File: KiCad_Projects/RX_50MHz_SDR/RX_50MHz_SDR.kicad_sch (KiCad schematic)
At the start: 0 parts

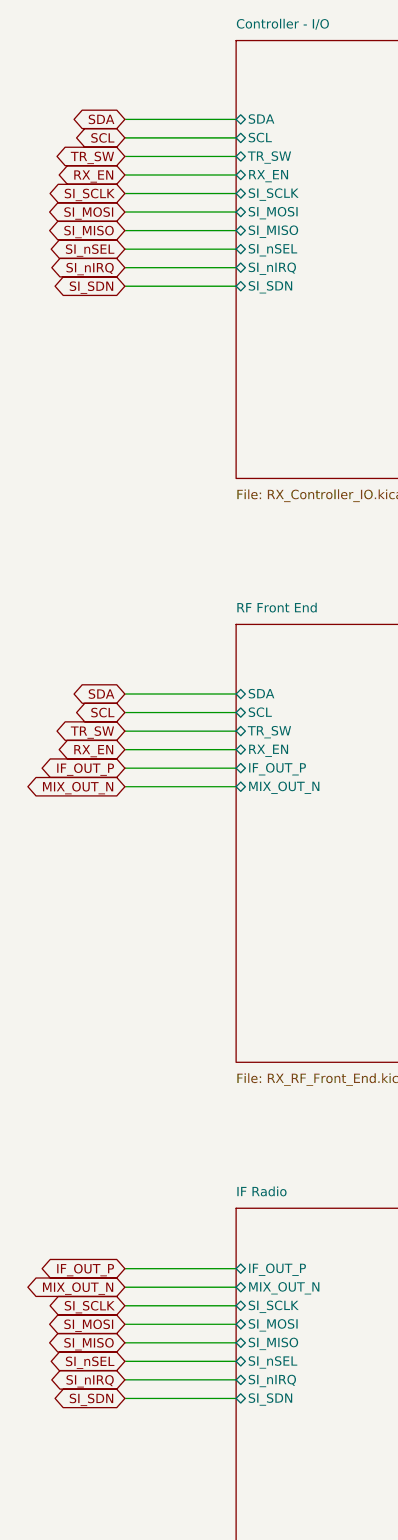
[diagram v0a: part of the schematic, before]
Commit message: lable correctly, local nets connected
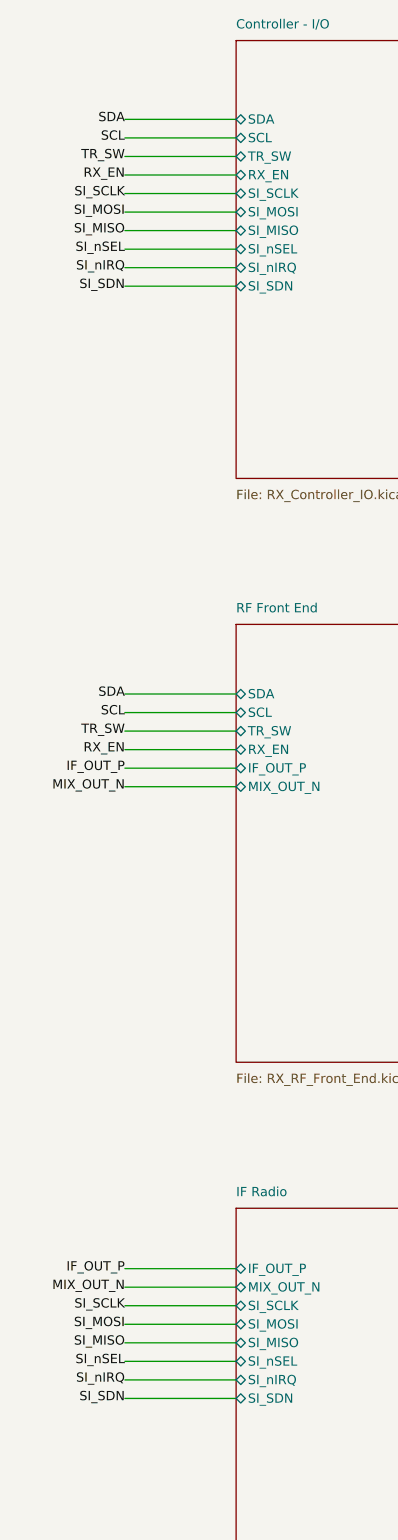
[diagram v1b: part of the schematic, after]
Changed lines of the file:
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@@
 	)
 	(wire (pts (xy 459.74 50.80) (xy 444.5 50.80)) (stroke (width 0) (type default)))
-	(global_label "SDA" (shape bidirectional) (at 444.5 50.80 180) (fields_autoplaced yes) (effects (font (size 1.27 1.27)) (justify right)))
+	(label "SDA"
+		(at 444.5 50.80 180)
+		(effects (font (size 1.27 1.27)) (justify right))
+	)
 	(wire (pts (xy 459.74 53.34) (xy 444.5 53.34)) (stroke (width 0) (type default)))
-	(global_label "SCL" (shape bidirectional) (at 444.5 53.34 180) (fields_autoplaced yes) (effects (font (size 1.27 1.27)) (justify right)))
+	(label "SCL"
+		(at 444.5 53.34 180)
+		(effects (font (size 1.27 1.27)) (justify right))
+	)
 	(wire (pts (xy 459.74 55.88) (xy 444.5 55.88)) (stroke (width 0) (type default)))
-	(global_label "TR_SW" (shape bidirectional) (at 444.5 55.88 180) (fields_autoplaced yes) (effects (font (size 1.27 1.27)) (justify right)))
+	(label "TR_SW"
+		(at 444.5 55.88 180)
+		(effects (font (size 1.27 1.27)) (justify right))
+	)
 	(wire (pts (xy 459.74 58.42) (xy 444.5 58.42)) (stroke (width 0) (type default)))
-	(global_label "RX_EN" (shape bidirectional) (at 444.5 58.42 180) (fields_autoplaced yes) (effects (font (size 1.27 1.27)) (justify right)))
+	(label "RX_EN"
+		(at 444.5 58.42 180)
+		(effects (font (size 1.27 1.27)) (justify right))
+	)
 	(wire (pts (xy 459.74 60.96) (xy 444.5 60.96)) (stroke (width 0) (type default)))
-	(global_label "SI_SCLK" (shape bidirectional) (at 444.5 60.96 180) (fields_autoplaced yes) (effects (font (size 1.27 1.27)) (justify right)))
+	(label "SI_SCLK"
+		(at 444.5 60.96 180)
+		(effects (font (size 1.27 1.27)) (justify right))
+	)
 	(wire (pts (xy 459.74 63.50) (xy 444.5 63.50)) (stroke (width 0) (type default)))
-	(global_label "SI_MOSI" (shape bidirectional) (at 444.5 63.50 180) (fields_autoplaced yes) (effects (font (size 1.27 1.27)) (justify right)))
+	(label "SI_MOSI"
+		(at 444.5 63.50 180)
+		(effects (font (size 1.27 1.27)) (justify right))
+	)
 	(wire (pts (xy 459.74 66.04) (xy 444.5 66.04)) (stroke (width 0) (type default)))
-	(global_label "SI_MISO" (shape bidirectional) (at 444.5 66.04 180) (fields_autoplaced yes) (effects (font (size 1.27 1.27)) (justify right)))
+	(label "SI_MISO"
+		(at 444.5 66.04 180)
+		(effects (font (size 1.27 1.27)) (justify right))
+	)
 	(wire (pts (xy 459.74 68.58) (xy 444.5 68.58)) (stroke (width 0) (type default)))
-	(global_label "SI_nSEL" (shape bidirectional) (at 444.5 68.58 180) (fields_autoplaced yes) (effects (font (size 1.27 1.27)) (justify right)))
+	(label "SI_nSEL"
+		(at 444.5 68.58 180)
+		(effects (font (size 1.27 1.27)) (justify right))
+	)
 	(wire (pts (xy 459.74 71.12) (xy 444.5 71.12)) (stroke (width 0) (type default)))
-	(global_label "SI_nIRQ" (shape bidirectional) (at 444.5 71.12 180) (fields_autoplaced yes) (effects (font (size 1.27 1.27)) (justify right)))
+	(label "SI_nIRQ"
+		(at 444.5 71.12 180)
+		(effects (font (size 1.27 1.27)) (justify right))
+	)
 	(wire (pts (xy 459.74 73.66) (xy 444.5 73.66)) (stroke (width 0) (type default)))
-	(global_label "SI_SDN" (shape bidirectional) (at 444.5 73.66 180) (fields_autoplaced yes) (effects (font (size 1.27 1.27)) (justify right)))
+	(label "SI_SDN"
+		(at 444.5 73.66 180)
+		(effects (font (size 1.27 1.27)) (justify right))
+	)
 	(wire (pts (xy 459.74 129.54) (xy 444.5 129.54)) (stroke (width 0) (type default)))
-	(global_label "SDA" (shape bidirectional) (at 444.5 129.54 180) (fields_autoplaced yes) (effects (font (size 1.27 1.27)) (justify right)))
+	(label "SDA"
+		(at 444.5 129.54 180)
+		(effects (font (size 1.27 1.27)) (justify right))
+	)
 	(wire (pts (xy 459.74 132.08) (xy 444.5 132.08)) (stroke (width 0) (type default)))
-	(global_label "SCL" (shape bidirectional) (at 444.5 132.08 180) (fields_autoplaced yes) (effects (font (size 1.27 1.27)) (justify right)))
+	(label "SCL"
+		(at 444.5 132.08 180)
+		(effects (font (size 1.27 1.27)) (justify right))
+	)
 	(wire (pts (xy 459.74 134.62) (xy 444.5 134.62)) (stroke (width 0) (type default)))
-	(global_label "TR_SW" (shape bidirectional) (at 444.5 134.62 180) (fields_autoplaced yes) (effects (font (size 1.27 1.27)) (justify right)))
+	(label "TR_SW"
+		(at 444.5 134.62 180)
+		(effects (font (size 1.27 1.27)) (justify right))
+	)
 	(wire (pts (xy 459.74 137.16) (xy 444.5 137.16)) (stroke (width 0) (type default)))
-	(global_label "RX_EN" (shape bidirectional) (at 444.5 137.16 180) (fields_autoplaced yes) (effects (font (size 1.27 1.27)) (justify right)))
+	(label "RX_EN"
+		(at 444.5 137.16 180)
+		(effects (font (size 1.27 1.27)) (justify right))
+	)
 	(wire (pts (xy 459.74 139.70) (xy 444.5 139.70)) (stroke (width 0) (type default)))
-	(global_label "IF_OUT_P" (shape bidirectional) (at 444.5 139.70 180) (fields_autoplaced yes) (effects (font (size 1.27 1.27)) (justify right)))
+	(label "IF_OUT_P"
+		(at 444.5 139.70 180)
+		(effects (font (size 1.27 1.27)) (justify right))
+	)
 	(wire (pts (xy 459.74 142.24) (xy 444.5 142.24)) (stroke (width 0) (type default)))
-	(global_label "MIX_OUT_N" (shape bidirectional) (at 444.5 142.24 180) (fields_autoplaced yes) (effects (font (size 1.27 1.27)) (justify right)))
+	(label "MIX_OUT_N"
+		(at 444.5 142.24 180)
+		(effects (font (size 1.27 1.27)) (justify right))
+	)
 	(wire (pts (xy 459.74 208.28) (xy 444.5 208.28)) (stroke (width 0) (type default)))
-	(global_label "IF_OUT_P" (shape bidirectional) (at 444.5 208.28 180) (fields_autoplaced yes) (effects (font (size 1.27 1.27)) (justify right)))
+	(label "IF_OUT_P"
+		(at 444.5 208.28 180)
+		(effects (font (size 1.27 1.27)) (justify right))
+	)
 	(wire (pts (xy 459.74 210.82) (xy 444.5 210.82)) (stroke (width 0) (type default)))
-	(global_label "MIX_OUT_N" (shape bidirectional) (at 444.5 210.82 180) (fields_autoplaced yes) (effects (font (size 1.27 1.27)) (justify right)))
+	(label "MIX_OUT_N"
+		(at 444.5 210.82 180)
+		(effects (font (size 1.27 1.27)) (justify right))
+	)
 	(wire (pts (xy 459.74 213.36) (xy 444.5 213.36)) (stroke (width 0) (type default)))
-	(global_label "SI_SCLK" (shape bidirectional) (at 444.5 213.36 180) (fields_autoplaced yes) (effects (font (size 1.27 1.27)) (justify right)))
+	(label "SI_SCLK"
+		(at 444.5 213.36 180)
+		(effects (font (size 1.27 1.27)) (justify right))
+	)
 	(wire (pts (xy 459.74 215.90) (xy 444.5 215.90)) (stroke (width 0) (type default)))
-	(global_label "SI_MOSI" (shape bidirectional) (at 444.5 215.90 180) (fields_autoplaced yes) (effects (font (size 1.27 1.27)) (justify right)))
+	(label "SI_MOSI"
+		(at 444.5 215.90 180)
+		(effects (font (size 1.27 1.27)) (justify right))
+	)
 	(wire (pts (xy 459.74 218.44) (xy 444.5 218.44)) (stroke (width 0) (type default)))
-	(global_label "SI_MISO" (shape bidirectional) (at 444.5 218.44 180) (fields_autoplaced yes) (effects (font (size 1.27 1.27)) (justify right)))
+	(label "SI_MISO"
+		(at 444.5 218.44 180)
+		(effects (font (size 1.27 1.27)) (justify right))
+	)
 	(wire (pts (xy 459.74 220.98) (xy 444.5 220.98)) (stroke (width 0) (type default)))
-	(global_label "SI_nSEL" (shape bidirectional) (at 444.5 220.98 180) (fields_autoplaced yes) (effects (font (size 1.27 1.27)) (justify right)))
+	(label "SI_nSEL"
+		(at 444.5 220.98 180)
+		(effects (font (size 1.27 1.27)) (justify right))
+	)
 	(wire (pts (xy 459.74 223.52) (xy 444.5 223.52)) (stroke (width 0) (type default)))
-	(global_label "SI_nIRQ" (shape bidirectional) (at 444.5 223.52 180) (fields_autoplaced yes) (effects (font (size 1.27 1.27)) (justify right)))
+	(label "SI_nIRQ"
+		(at 444.5 223.52 180)
+		(effects (font (size 1.27 1.27)) (justify right))
+	)
 	(wire (pts (xy 459.74 226.06) (xy 444.5 226.06)) (stroke (width 0) (type default)))
-	(global_label "SI_SDN" (shape bidirectional) (at 444.5 226.06 180) (fields_autoplaced yes) (effects (font (size 1.27 1.27)) (justify right)))(sheet_instances
+	(label "SI_SDN"
+		(at 444.5 226.06 180)
+		(effects (font (size 1.27 1.27)) (justify right))
+	)(sheet_instances
 		(path "/"
 			(page "1")
